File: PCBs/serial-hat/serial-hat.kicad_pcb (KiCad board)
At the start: 2 copper layers, 65 x 56 mm, 15 parts, among them CN1 Modem port, CN2 Printer port, J1 Conn_01x02_Pin, J7 Rpi headers, U1 PC817C-S, U2 MAX3232

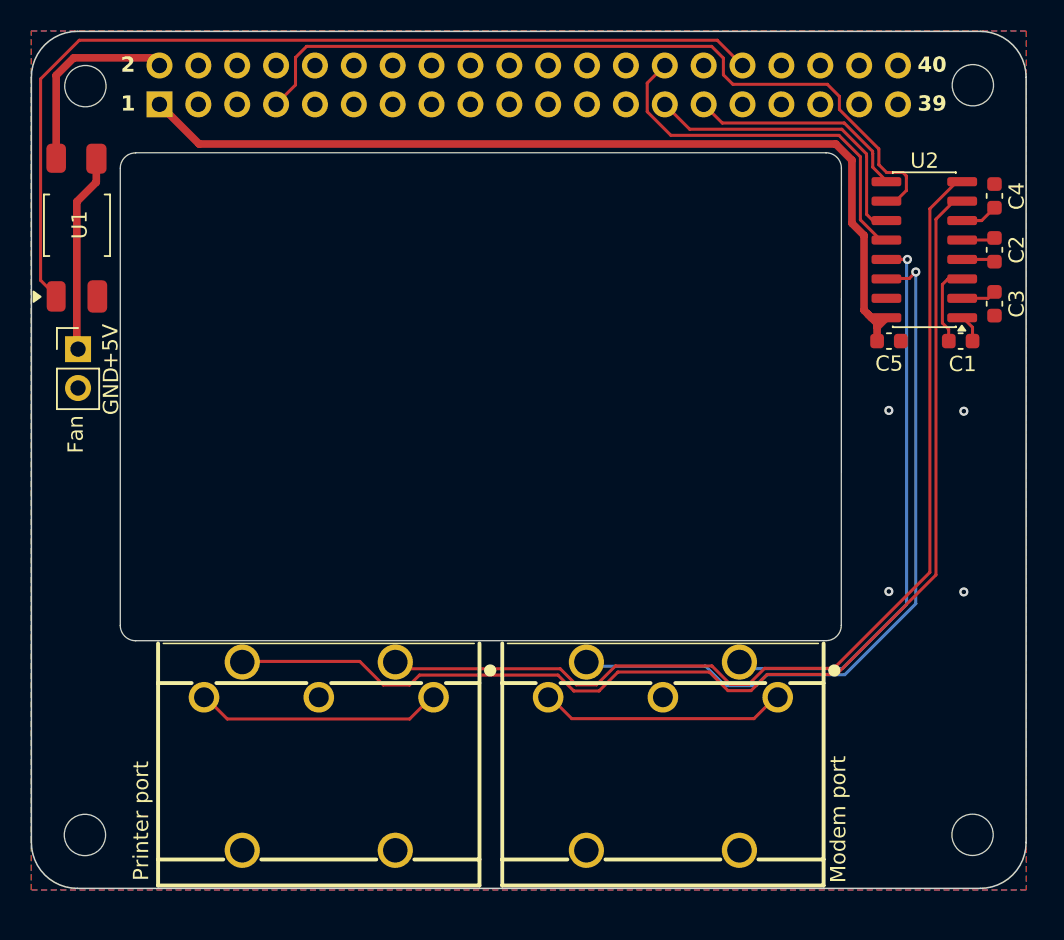
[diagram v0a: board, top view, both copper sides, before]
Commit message: Update stls and notes
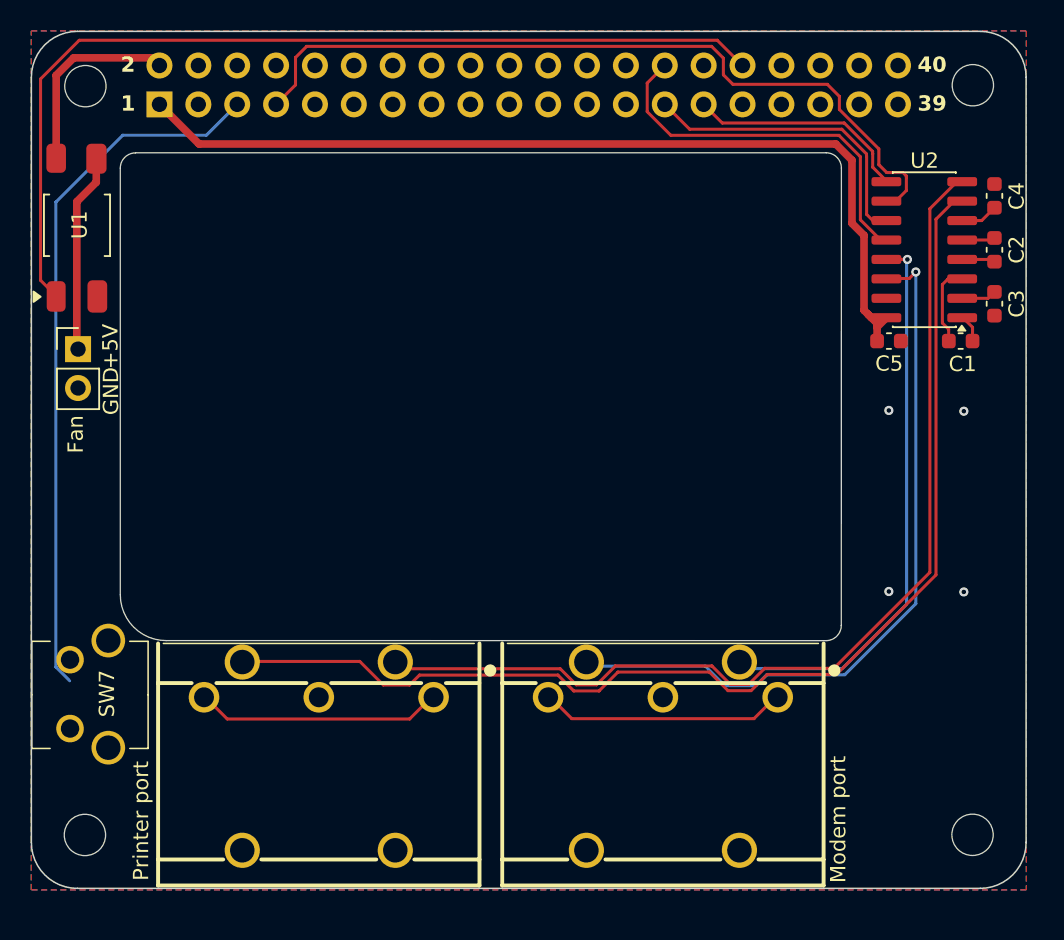
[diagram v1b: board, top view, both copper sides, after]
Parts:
- added SW7: SW_SPST, Colins-Kicad:SPST momentary switch C6575016, F.Cu at (127.8, 96.0)
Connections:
- J7 pad 5: unconnected-(J7-Pin_5-Pad5) -> PWR_BTN
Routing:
- net PWR_BTN: track 0.00 -> 46.1 mm
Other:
- outline, holes or cut-outs redrawn
